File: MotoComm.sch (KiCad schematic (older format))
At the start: 37 parts, among them J1 PGRM, J2 Audio-Jack-3, J3 Conn_01x03, J4 Conn_02x01, J5 USB_OTG, SW1 SW_Vol+, SW2 SW_Vol-, SW3 SW_NEXT, SW4 SW_PREV, SW5 SW_P_P_Call, SW6 SW_POWER, U1 LM358, U2 F-3188_CSR8645, U3 LT6656**S6

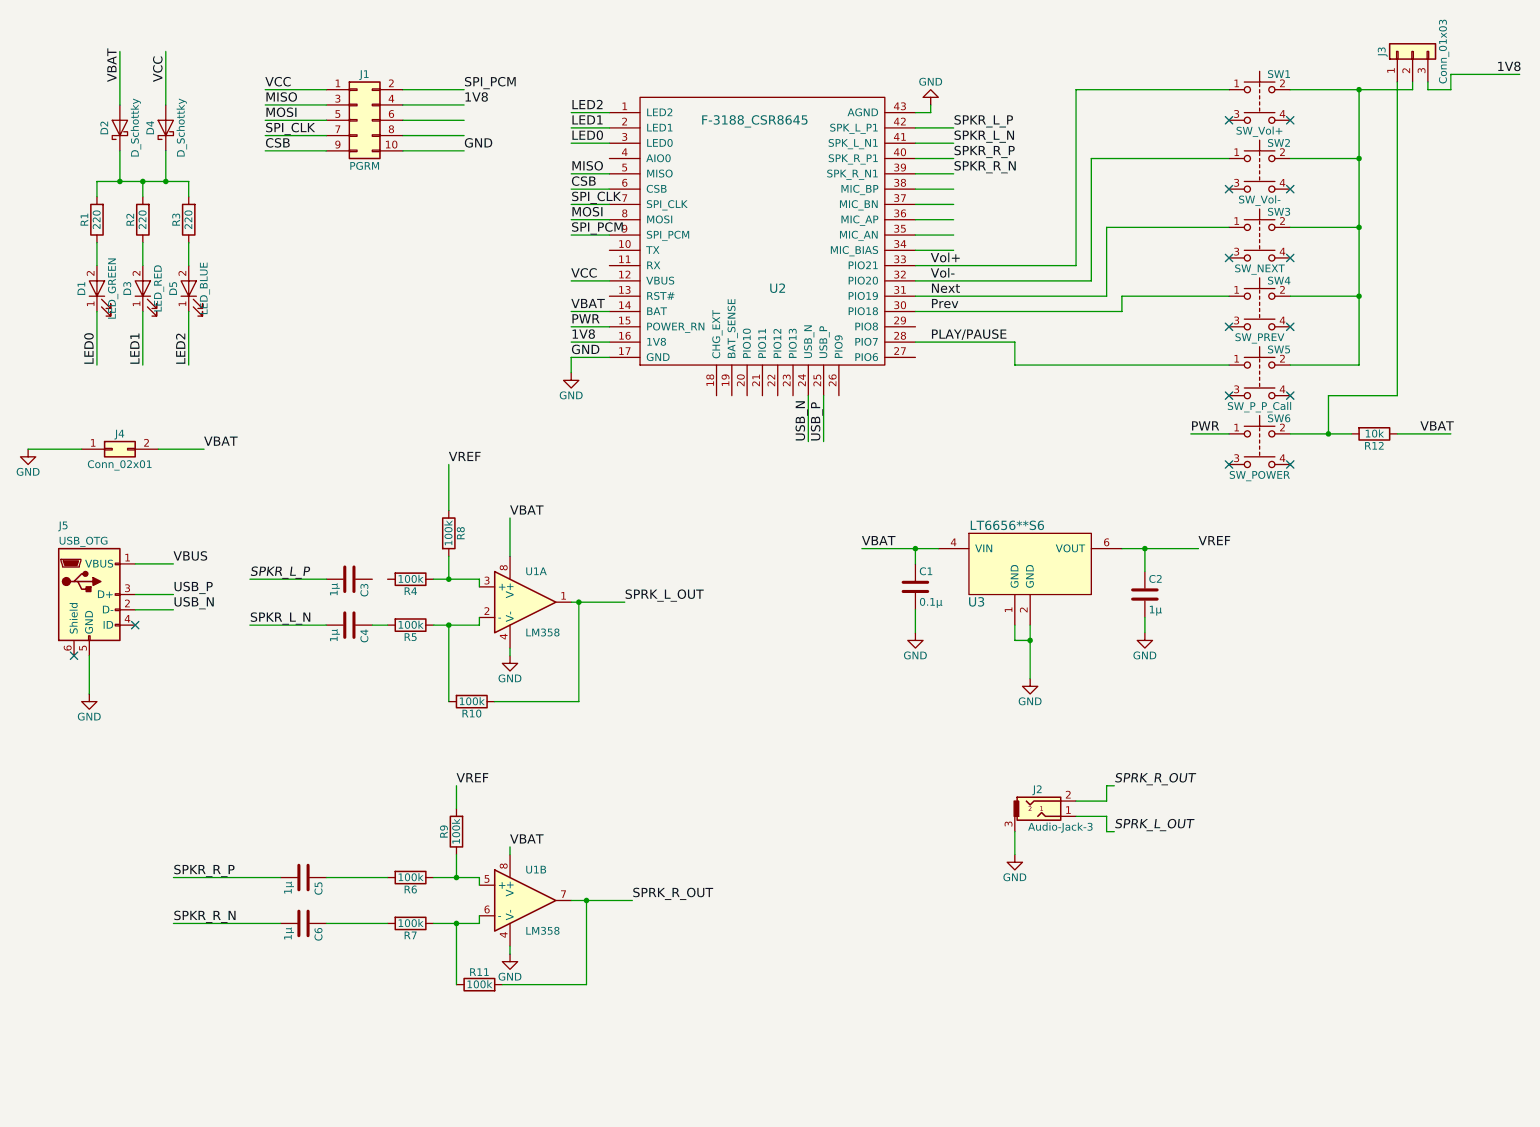
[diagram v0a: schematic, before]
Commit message: minor update
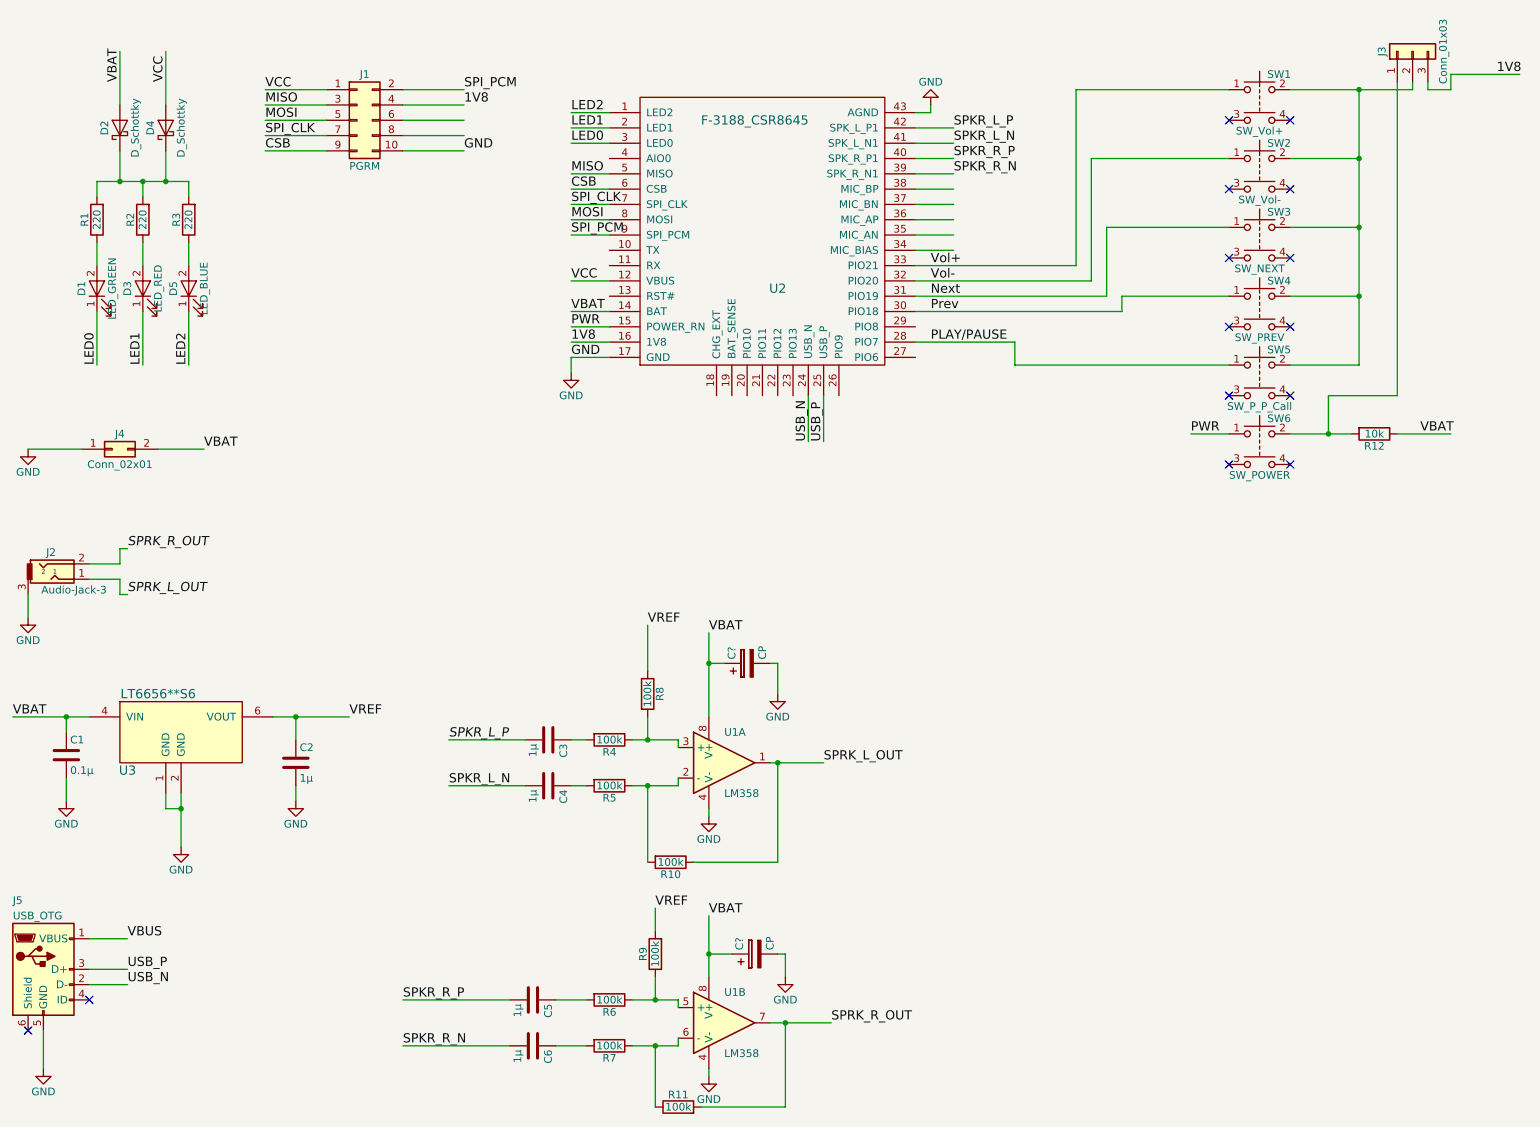
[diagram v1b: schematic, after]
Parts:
- added C? (x2): CP, symbol CP
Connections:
- wire segments 136 -> 143
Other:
- moved on the sheet: C1, C2, C3, C4, C5, C6, J2, J5, R10, R11, R4, R5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
